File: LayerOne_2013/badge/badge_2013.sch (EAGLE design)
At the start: 125 parts, among them CON2 EXT, CON6 J8, CON8 J3, IC1 SLICE_NOSHIFT_TLC5947HTSSOP32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, IC3 SLICE_NOSHIFT_TLC5947HTSSOP32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, IC4 TL064D, K1 5-XX, K2 5-XX, K3 5-XX, K4 5-XX, U1 UG-2864HSWEG01, U2 AP7333-33SOT23-3, U4 TPS60403, X2 NX3225GA

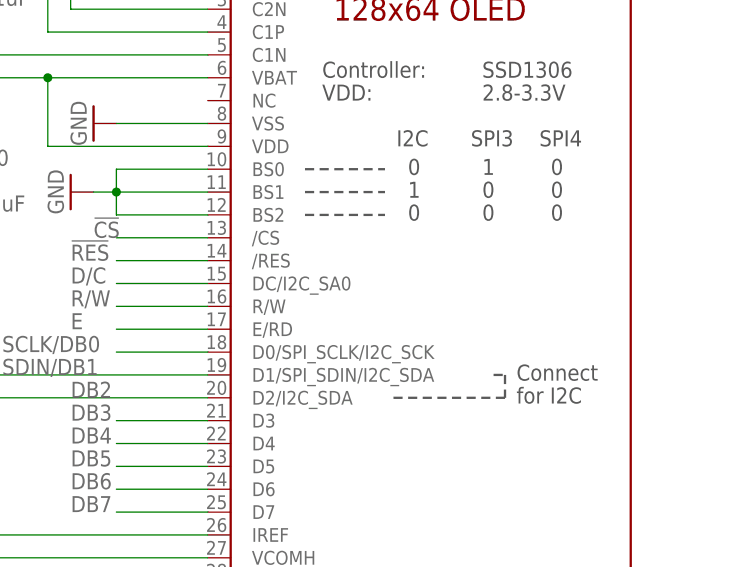
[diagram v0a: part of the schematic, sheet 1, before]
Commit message: oled update
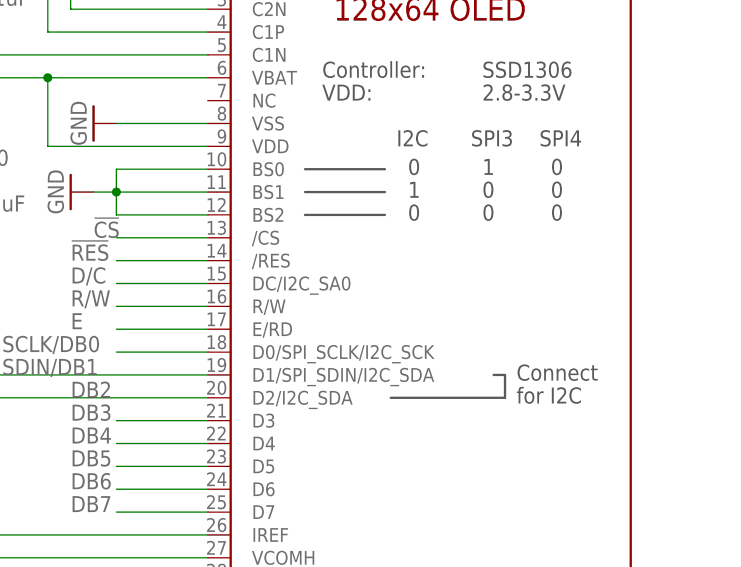
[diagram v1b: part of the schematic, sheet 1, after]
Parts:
- SJ1: device microbuilder:SOLDERJUMPERREFLOW_NOPASTE -> microbuilder:SOLDERJUMPERREFLOW
- U1: device microbuilder:DISP_OLED_UG-2864HSWEG010.96" -> badge.lbrbadge_2013:MICROBUILDER_DISP_OLED_UG-2864HSWEG010.96"
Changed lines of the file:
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@@
 <part name="BAT1" library="tvbgone-adj" deviceset="BATTERY" device="CR123A" value="CR123A"/>
 <part name="GND6" library="supply1" deviceset="GND" device=""/>
-<part name="U1" library="microbuilder" deviceset="DISP_OLED_UG-2864HSWEG01" device="0.96&quot;" value="UG-2864HSWEG01"/>
+<part name="U1" library="badge.lbrbadge_2013" deviceset="MICROBUILDER_DISP_OLED_UG-2864HSWEG01" device="0.96&quot;" value="UG-2864HSWEG01"/>
 <part name="C14" library="SparkFun" deviceset="CAP" device="0805" value="1uF"/>
 <part name="GND3" library="SparkFun" deviceset="GND" device=""/>
@@
 <part name="GND47" library="SparkFun" deviceset="GND" device=""/>
 <part name="JP1" library="microbuilder" deviceset="JUMPER3" device=""/>
-<part name="SJ1" library="microbuilder" deviceset="SOLDERJUMPER" device="REFLOW_NOPASTE"/>
+<part name="SJ1" library="microbuilder" deviceset="SOLDERJUMPER" device="REFLOW"/>
 <part name="R24" library="resistor" deviceset="R-US_" device="R0805" value="3K"/>
 <part name="PDI" library="microbuilder" deviceset="HEADER-1X2" device="" value="CON6"/>
